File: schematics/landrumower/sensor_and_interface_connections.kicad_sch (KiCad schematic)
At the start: 11 parts, among them J11 UART, J12 BumperY, J13 BumperX, J14 I2C0, J15 Lift, J16 StopButton, J17 I2C1, J18 Rain, J19 ResrveGPIO/ADC0, J20 ReserveGPIO, J21 ReserveGPIO/ADC1

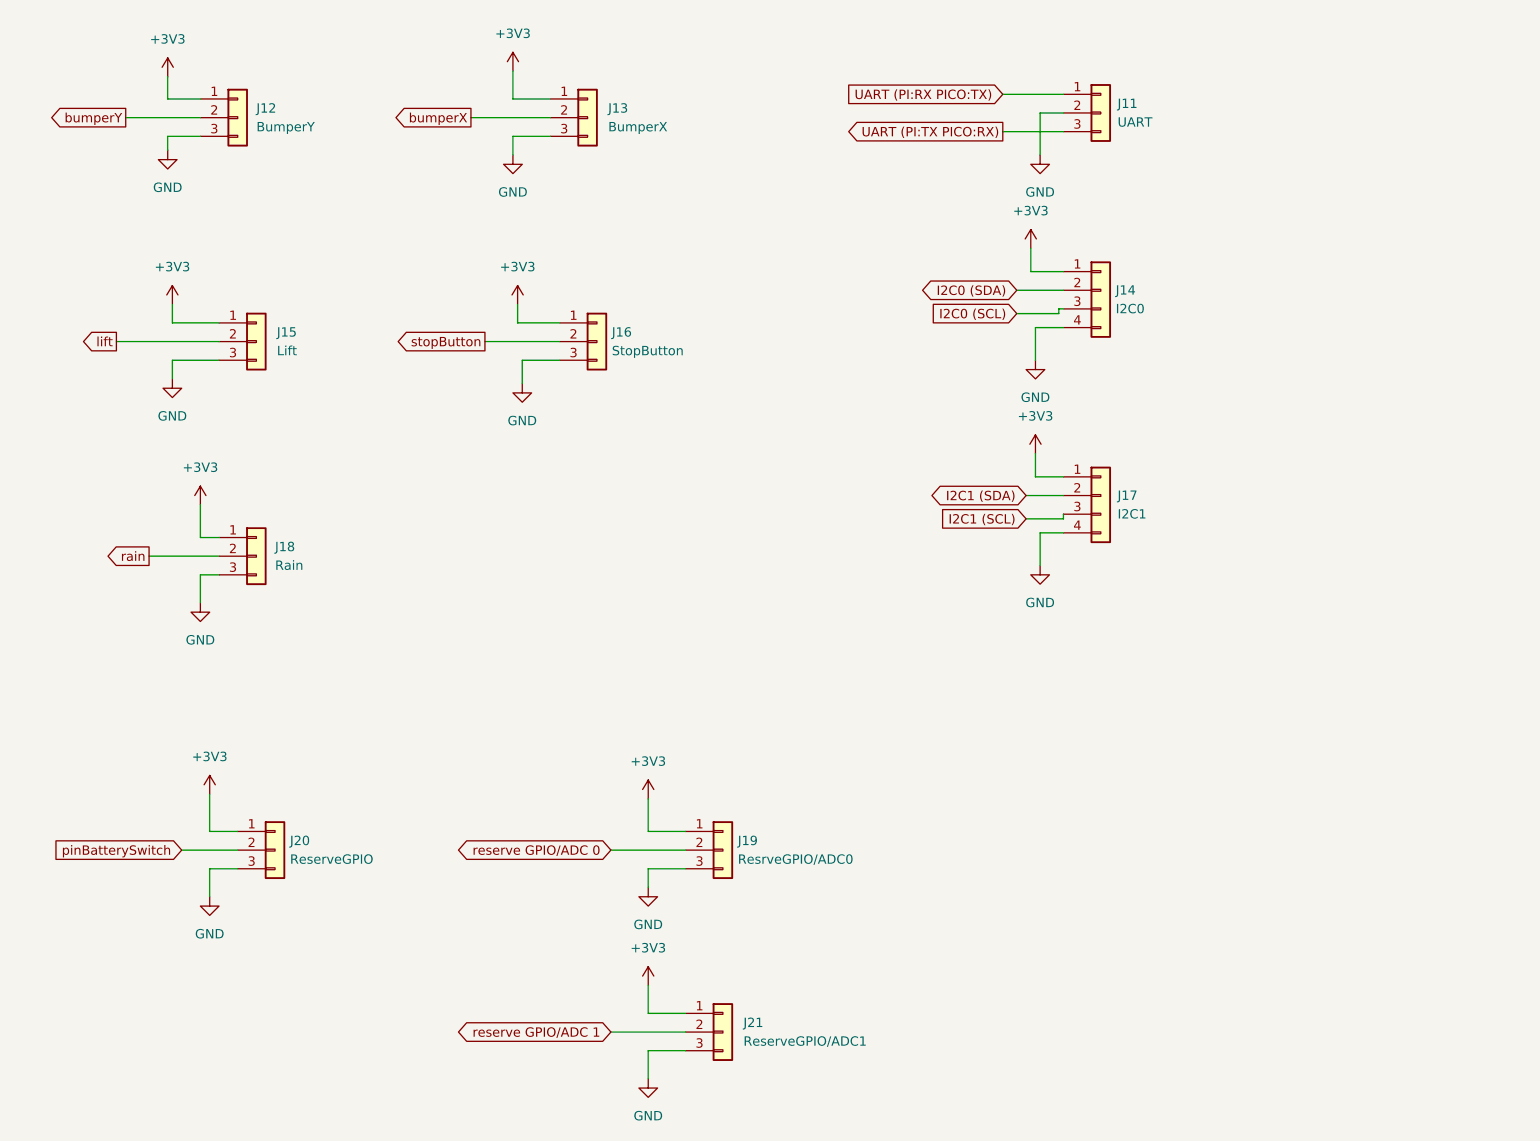
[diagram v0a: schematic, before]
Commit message: PCB changes for Landrumower
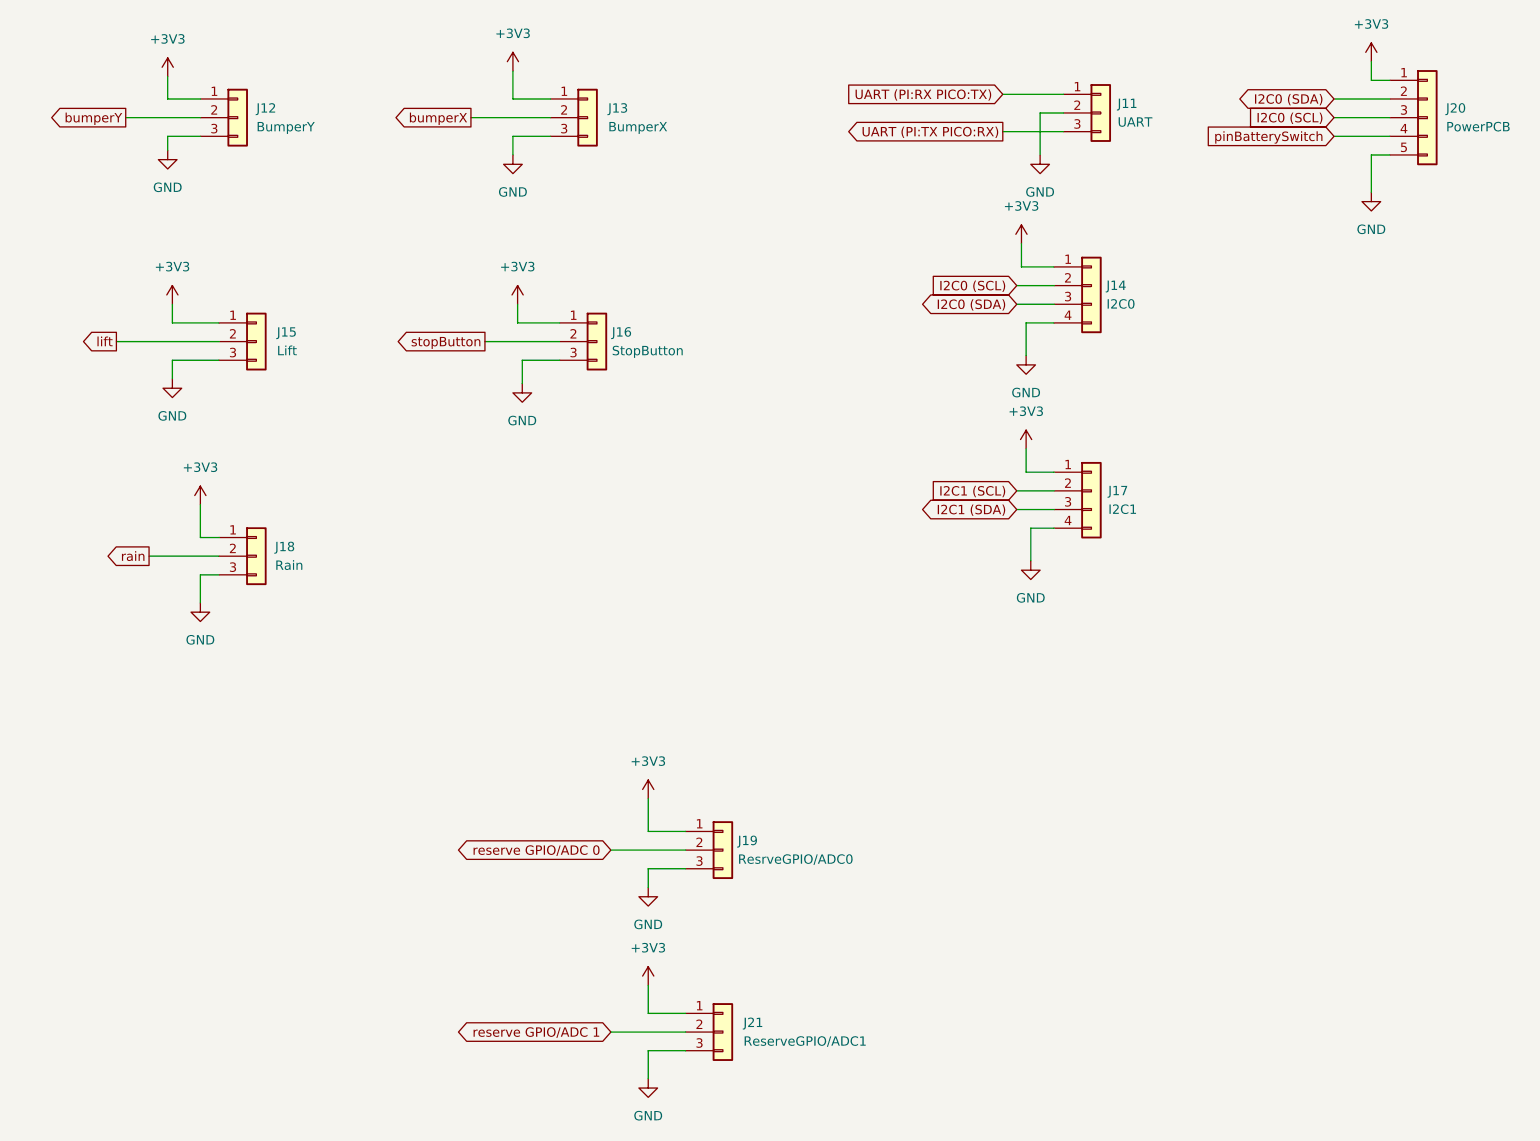
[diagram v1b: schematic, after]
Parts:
- removed J20: ReserveGPIO, Connector_JST:JST_EH_B3B-EH-A_1x03_P2.50mm_Vertical, symbol Connector_Generic:Conn_01x03
- added J20: PowerPCB, Connector_JST:JST_EH_B5B-EH-A_1x05_P2.50mm_Vertical, symbol Connector_Generic:Conn_01x05
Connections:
- net +3V3: now also J20.1 (Pin_1)
- net GND: now also J20.5 (Pin_5)
- net I2C0 (SCL): now also J14.2 (Pin_2), J20.3 (Pin_3); no longer J14.3 (Pin_3)
- net I2C0 (SDA): now also J14.3 (Pin_3), J20.2 (Pin_2); no longer J14.2 (Pin_2)
- net I2C1 (SCL): now also J17.2 (Pin_2); no longer J17.3 (Pin_3)
- net I2C1 (SDA): now also J17.3 (Pin_3); no longer J17.2 (Pin_2)
- net pinBatterySwitch: now also J20.4 (Pin_4)
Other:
- moved on the sheet: J14, J17
